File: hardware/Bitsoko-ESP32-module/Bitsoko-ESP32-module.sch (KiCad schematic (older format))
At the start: 0 parts

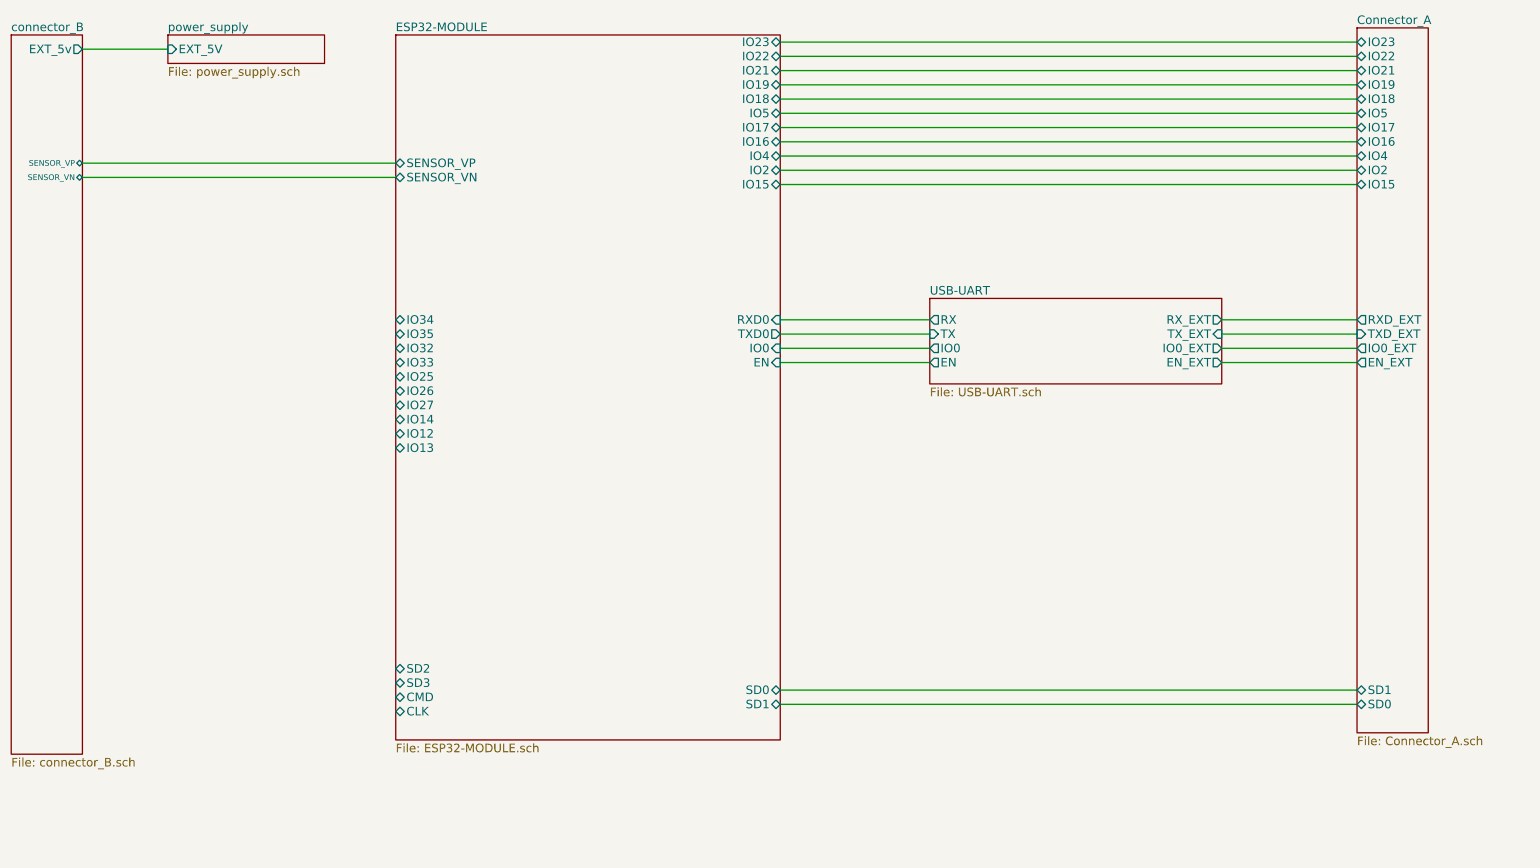
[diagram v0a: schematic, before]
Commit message: Semicomplete Bitsoko ESP32 module
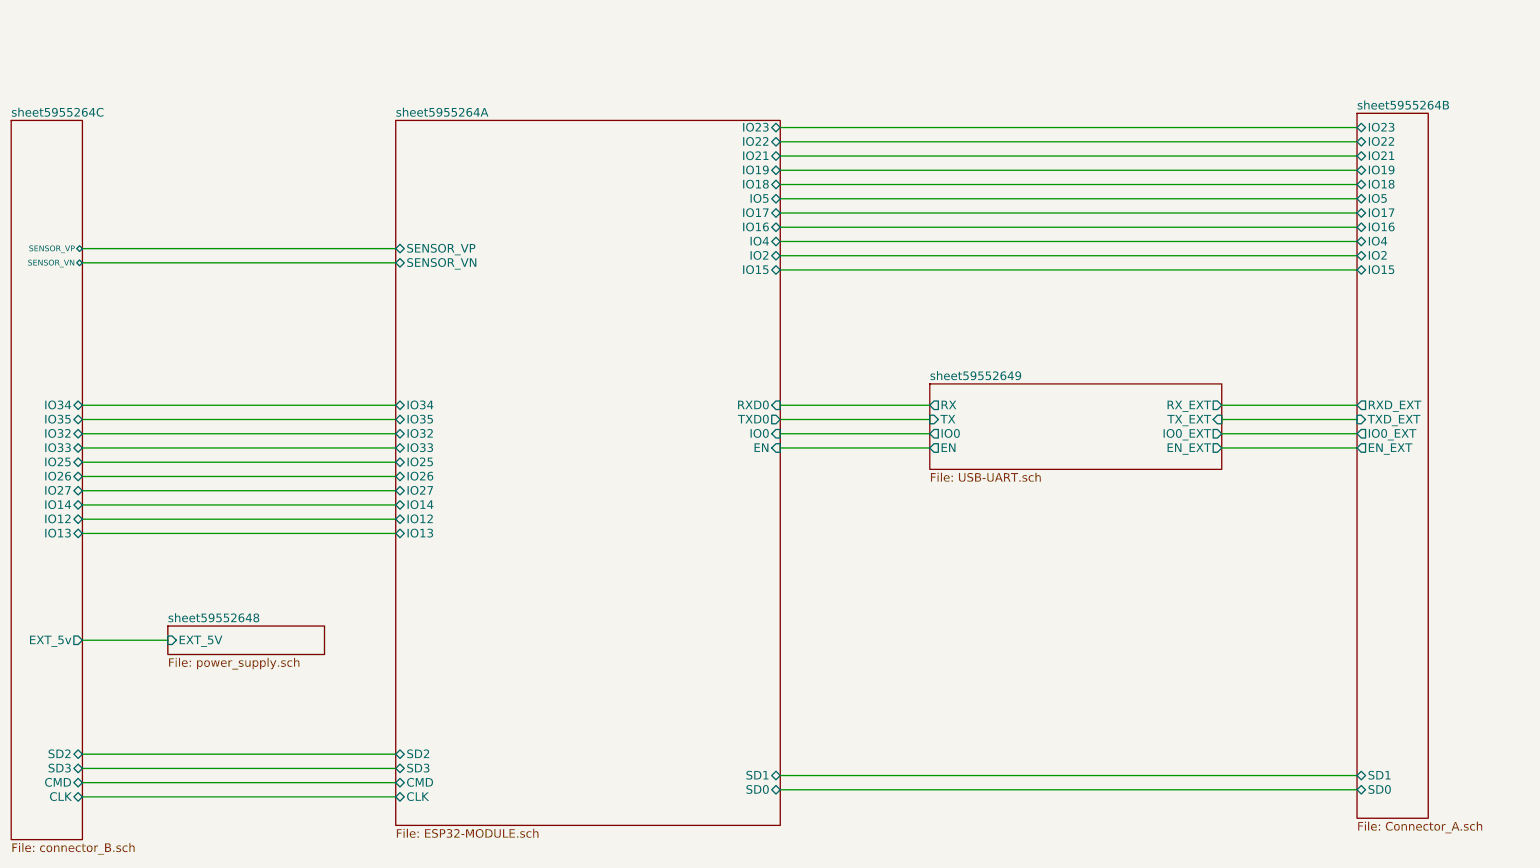
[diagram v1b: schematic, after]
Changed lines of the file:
@@
 $EndDescr
 $Sheet
-S 1850 900  1100 200
-U 59510B2B
-F0 "power_supply" 60
+S 1850 5050 1100 200
+U 5955264F
+F0 "sheet59552648" 60
 F1 "power_supply.sch" 60
-F2 "EXT_5V" I L 1850 1000 60
+F2 "EXT_5V" I L 1850 5150 60
 $EndSheet
 $Sheet
-S 7200 2750 2050 600
-U 59510B33
-F0 "USB-UART" 60
+S 7200 3350 2050 600
+U 5955265C
+F0 "sheet59552649" 60
 F1 "USB-UART.sch" 60
-F2 "RX" O L 7200 2900 60
-F3 "TX" I L 7200 3000 60
-F4 "IO0" O L 7200 3100 60
-F5 "EN" O L 7200 3200 60
-F6 "RX_EXT" O R 9250 2900 60
-F7 "TX_EXT" I R 9250 3000 60
-F8 "IO0_EXT" O R 9250 3100 60
-F9 "EN_EXT" O R 9250 3200 60
+F2 "RX" O L 7200 3500 60
+F3 "TX" I L 7200 3600 60
+F4 "IO0" O L 7200 3700 60
+F5 "EN" O L 7200 3800 60
+F6 "RX_EXT" O R 9250 3500 60
+F7 "TX_EXT" I R 9250 3600 60
+F8 "IO0_EXT" O R 9250 3700 60
+F9 "EN_EXT" O R 9250 3800 60
 $EndSheet
 $Sheet
-S 3450 900  2700 4950
-U 59510B38
-F0 "ESP32-MODULE" 60
+S 3450 1500 2700 4950
+U 59552697
+F0 "sheet5955264A" 60
 F1 "ESP32-MODULE.sch" 60
-F2 "EN" I R 6150 3200 60
-F3 "IO23" B R 6150 950 60
-F4 "IO22" B R 6150 1050 60
-F5 "TXD0" O R 6150 3000 60
-F6 "RXD0" I R 6150 2900 60
-F7 "IO21" B R 6150 1150 60
-F8 "IO19" B R 6150 1250 60
-F9 "IO18" B R 6150 1350 60
-F10 "IO5" B R 6150 1450 60
-F11 "IO17" B R 6150 1550 60
-F12 "IO16" B R 6150 1650 60
-F13 "IO4" B R 6150 1750 60
-F14 "IO2" B R 6150 1850 60
-F15 "IO15" B R 6150 1950 60
-F16 "SD1" B R 6150 5600 60
-F17 "SD0" B R 6150 5500 60
-F18 "CLK" B L 3450 5650 60
-F19 "CMD" B L 3450 5550 60
-F20 "SD3" B L 3450 5450 60
-F21 "SD2" B L 3450 5350 60
-F22 "IO13" B L 3450 3800 60
-F23 "IO12" B L 3450 3700 60
-F24 "IO14" B L 3450 3600 60
-F25 "IO27" B L 3450 3500 60
-F26 "IO26" B L 3450 3400 60
-F27 "IO25" B L 3450 3300 60
-F28 "IO33" B L 3450 3200 60
-F29 "IO32" B L 3450 3100 60
-F30 "IO35" B L 3450 3000 60
-F31 "IO34" B L 3450 2900 60
-F32 "SENSOR_VN" B L 3450 1900 60
-F33 "SENSOR_VP" B L 3450 1800 60
-F34 "IO0" I R 6150 3100 60
+F2 "EN" I R 6150 3800 60
+F3 "IO23" B R 6150 1550 60
+F4 "IO22" B R 6150 1650 60
+F5 "TXD0" O R 6150 3600 60
+F6 "RXD0" I R 6150 3500 60
+F7 "IO21" B R 6150 1750 60
+F8 "IO19" B R 6150 1850 60
+F9 "IO18" B R 6150 1950 60
+F10 "IO5" B R 6150 2050 60
+F11 "IO17" B R 6150 2150 60
+F12 "IO16" B R 6150 2250 60
+F13 "IO4" B R 6150 2350 60
+F14 "IO2" B R 6150 2450 60
+F15 "IO15" B R 6150 2550 60
+F16 "SD1" B R 6150 6100 60
+F17 "SD0" B R 6150 6200 60
+F18 "CLK" B L 3450 6250 60
+F19 "CMD" B L 3450 6150 60
+F20 "SD3" B L 3450 6050 60
+F21 "SD2" B L 3450 5950 60
+F22 "IO13" B L 3450 4400 60
+F23 "IO12" B L 3450 4300 60
+F24 "IO14" B L 3450 4200 60
+F25 "IO27" B L 3450 4100 60
+F26 "IO26" B L 3450 4000 60
+F27 "IO25" B L 3450 3900 60
+F28 "IO33" B L 3450 3800 60
+F29 "IO32" B L 3450 3700 60
+F30 "IO35" B L 3450 3600 60
+F31 "IO34" B L 3450 3500 60
+F32 "SENSOR_VN" B L 3450 2500 60
+F33 "SENSOR_VP" B L 3450 2400 60
+F34 "IO0" I R 6150 3700 60
 $EndSheet
 $Sheet
-S 10200 850  500  4950
-U 59510B3D
-F0 "Connector_A" 60
+S 10200 1450 500  4950
+U 5955270D
+F0 "sheet5955264B" 60
 F1 "Connector_A.sch" 60
-F2 "IO23" B L 10200 950 60
-F3 "IO22" B L 10200 1050 60
-F4 "IO21" B L 10200 1150 60
-F5 "IO19" B L 10200 1250 60
-F6 "IO18" B L 10200 1350 60
-F7 "IO5" B L 10200 1450 60
-F8 "IO17" B L 10200 1550 60
-F9 "IO16" B L 10200 1650 60
-F10 "IO4" B L 10200 1750 60
-F11 "IO2" B L 10200 1850 60
-F12 "IO15" B L 10200 1950 60
-F13 "RXD_EXT" O L 10200 2900 60
-F14 "TXD_EXT" I L 10200 3000 60
-F15 "IO0_EXT" O L 10200 3100 60
-F16 "EN_EXT" O L 10200 3200 60
-F17 "SD1" B L 10200 5500 60
-F18 "SD0" B L 10200 5600 60
+F2 "IO23" B L 10200 1550 60
+F3 "IO22" B L 10200 1650 60
+F4 "IO21" B L 10200 1750 60
+F5 "IO19" B L 10200 1850 60
+F6 "IO18" B L 10200 1950 60
+F7 "IO5" B L 10200 2050 60
+F8 "IO17" B L 10200 2150 60
+F9 "IO16" B L 10200 2250 60
+F10 "IO4" B L 10200 2350 60
+F11 "IO2" B L 10200 2450 60
+F12 "IO15" B L 10200 2550 60
+F13 "RXD_EXT" O L 10200 3500 60
+F14 "TXD_EXT" I L 10200 3600 60
+F15 "IO0_EXT" O L 10200 3700 60
+F16 "EN_EXT" O L 10200 3800 60
+F17 "SD1" B L 10200 6100 60
+F18 "SD0" B L 10200 6200 60
 $EndSheet
 $Sheet
-S 750  900  500  5050
-U 59510C04
-F0 "connector_B" 60
+S 750  1500 500  5050
+U 59552753
+F0 "sheet5955264C" 60
 F1 "connector_B.sch" 60
-F2 "EXT_5v" O R 1250 1000 60
-F3 "SENSOR_VP" B R 1250 1800 40
-F4 "SENSOR_VN" B R 1250 1900 40
+F2 "EXT_5v" O R 1250 5150 60
+F3 "SENSOR_VP" B R 1250 2400 40
+F4 "SENSOR_VN" B R 1250 2500 40
+F5 "IO34" B R 1250 3500 60
+F6 "IO35" B R 1250 3600 60
+F7 "IO32" B R 1250 3700 60
+F8 "IO33" B R 1250 3800 60
+F9 "IO25" B R 1250 3900 60
+F10 "IO26" B R 1250 4000 60
+F11 "IO27" B R 1250 4100 60
+F12 "IO14" B R 1250 4200 60
+F13 "IO12" B R 1250 4300 60
+F14 "IO13" B R 1250 4400 60
+F15 "SD2" B R 1250 5950 60
+F16 "SD3" B R 1250 6050 60
+F17 "CMD" B R 1250 6150 60
+F18 "CLK" B R 1250 6250 60
 $EndSheet
 Wire Wire Line
-	6150 2900 7200 2900
+	6150 3500 7200 3500
 Wire Wire Line
-	7200 3000 6150 3000
+	7200 3600 6150 3600
 Wire Wire Line
-	7200 3100 6150 3100
+	7200 3700 6150 3700
 Wire Wire Line
-	7200 3200 6150 3200
-Wire Wire Line
-	10200 950  6150 950
-Wire Wire Line
-	10200 1050 6150 1050
-Wire Wire Line
-	10200 1150 6150 1150
-Wire Wire Line
-	10200 1250 6150 1250
-Wire Wire Line
-	10200 1350 6150 1350
-Wire Wire Line
-	10200 1450 6150 1450
+	7200 3800 6150 3800
 Wire Wire Line
 	10200 1550 6150 1550
@@
 	10200 1950 6150 1950
 Wire Wire Line
-	9250 2900 10200 2900
+	10200 2050 6150 2050
 Wire Wire Line
-	9250 3000 10200 3000
+	10200 2150 6150 2150
 Wire Wire Line
-	9250 3100 10200 3100
+	10200 2250 6150 2250
 Wire Wire Line
-	9250 3200 10200 3200
+	10200 2350 6150 2350
 Wire Wire Line
-	10200 5500 6150 5500
+	10200 2450 6150 2450
 Wire Wire Line
-	10200 5600 6150 5600
+	10200 2550 6150 2550
 Wire Wire Line
-	1250 1000 1850 1000
+	9250 3500 10200 3500
 Wire Wire Line
-	3450 1800 1250 1800
+	9250 3600 10200 3600
 Wire Wire Line
-	3450 1900 1250 1900
+	9250 3700 10200 3700
+Wire Wire Line
+	9250 3800 10200 3800
+Wire Wire Line
+	10200 6100 6150 6100
+Wire Wire Line
+	10200 6200 6150 6200
+Wire Wire Line
+	1250 5150 1850 5150
+Wire Wire Line
+	3450 2400 1250 2400
+Wire Wire Line
+	3450 2500 1250 2500
+Wire Wire Line
+	1250 3500 3450 3500
+Wire Wire Line
+	1250 3600 3450 3600
+Wire Wire Line
+	1250 3700 3450 3700
+Wire Wire Line
+	1250 3800 3450 3800
+Wire Wire Line
+	1250 3900 3450 3900
+Wire Wire Line
+	1250 4000 3450 4000
+Wire Wire Line
+	1250 4100 3450 4100
+Wire Wire Line
+	1250 4200 3450 4200
+Wire Wire Line
+	1250 4300 3450 4300
+Wire Wire Line
+	1250 4400 3450 4400
+Wire Wire Line
+	3450 5950 1250 5950
+Wire Wire Line
+	3450 6050 1250 6050
+Wire Wire Line
+	3450 6150 1250 6150
+Wire Wire Line
+	3450 6250 1250 6250
 $EndSCHEMATC
